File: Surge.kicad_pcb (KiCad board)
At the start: 2 copper layers, 62.6 x 33.4 mm, 16 parts, among them SW1 C1005B 10A TCB

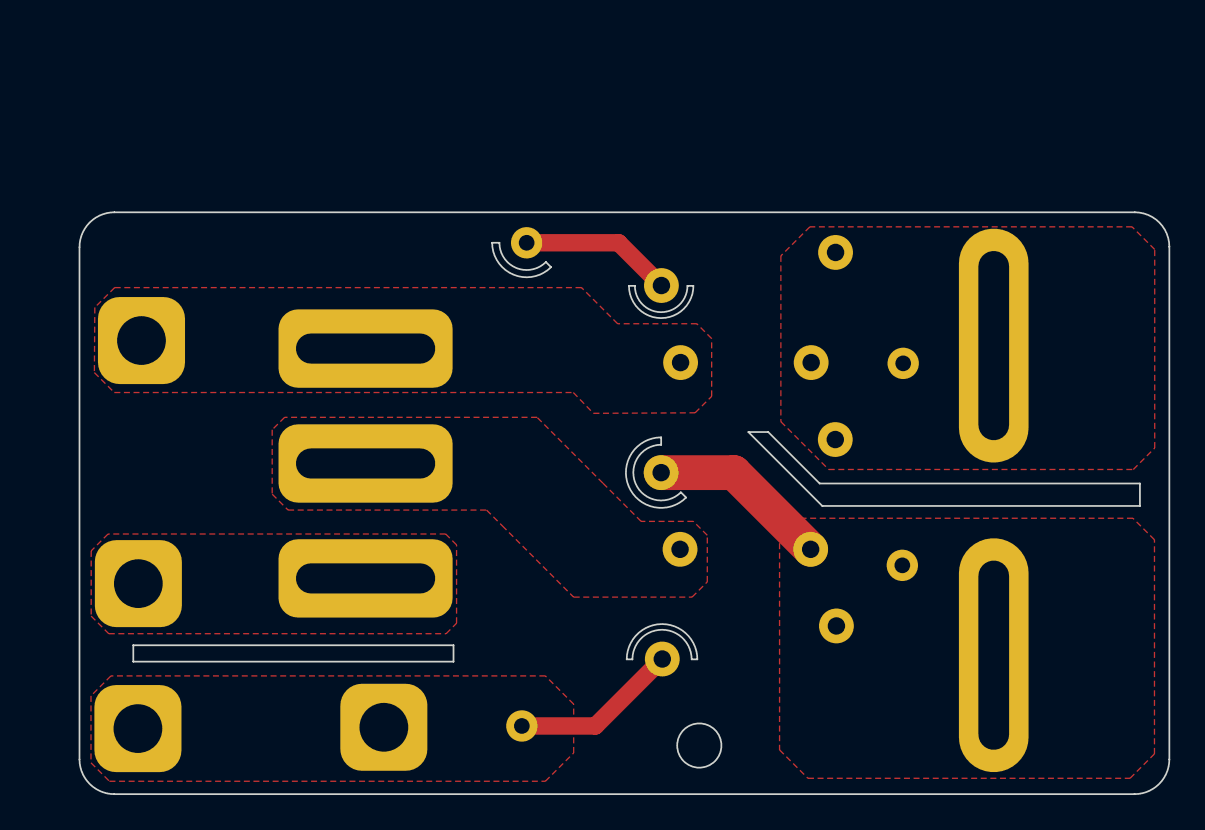
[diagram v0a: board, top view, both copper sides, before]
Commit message: update layout
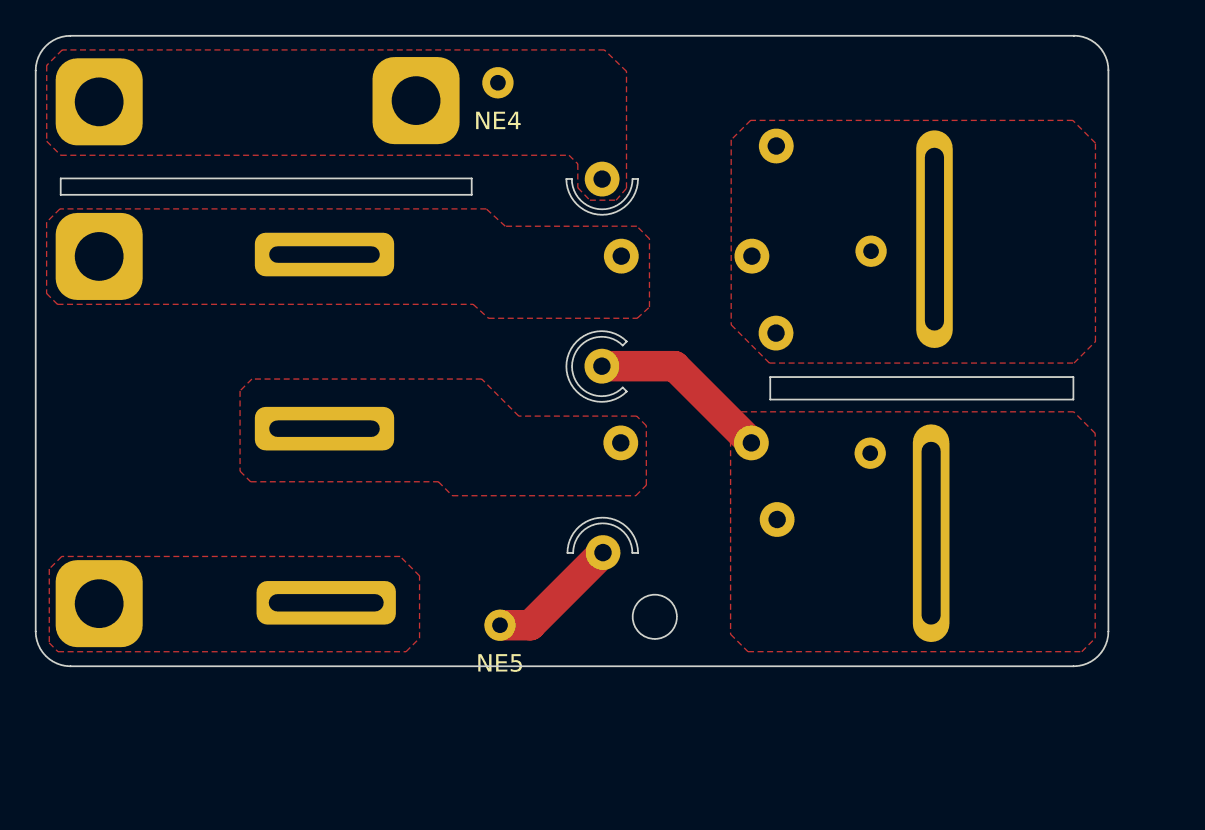
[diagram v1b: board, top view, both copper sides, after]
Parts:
- removed NE6: E_E, Surge_Library:NEmount
- added NE4: , Surge_Library:NEmount, F.Cu at (59.9, 31.2)
- NE5: value E_MOV -> (none)
- SW1: moved to B.Cu
- moved H3 36.1 mm to (36.4, 34.3)
- moved H6 36.0 mm to (59.9, 29.5)
- moved NE5 22.0 mm to (60.0, 62.3)
- moved H5 7.88 mm to (84.8, 62.0)
- moved H4 7.00 mm to (85.0, 45.1)
- moved F1 7.00 mm to (74.5, 38.4)
- moved F2 7.00 mm to (74.5, 49.2)
- moved RV1 7.00 mm to (65.9, 34.0)
- moved RV2 7.00 mm to (65.9, 44.8)
- moved RV3 7.00 mm to (75.9, 53.6)
- moved NE3 6.70 mm to (81.3, 52.5)
- moved NE2 6.70 mm to (81.3, 40.9)
- moved H1 5.38 mm to (37.1, 43.2)
- moved SW1 3.09 mm to (49.9, 48.4), turned to 180 degrees
- moved H2 2.92 mm to (36.6, 63.1)
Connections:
- RV1 pad 2: Net-(NE5-Pad1) -> Earth
- RV3 pad 2: Earth -> Net-(NE5-Pad1)
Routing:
- net Earth: track 9.66 -> 0.00 mm
- net Net-(NE5-Pad1): track 8.76 -> 7.64 mm
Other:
- board size 62.6 x 33.4 mm -> 61.6 x 36.2 mm
- board text added: "TCB"
- board text removed: "SPST_Neon SW"
